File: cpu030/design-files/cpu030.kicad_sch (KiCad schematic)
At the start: 67 parts, among them J101 Reset, J102 SYSCTL JTAG, J103 NMI, SW101 Reset, SW102 NMI, U101 MC68030RC, U102 ATF1508AS, U103 74ACT05, U104 DS1813, U105 SST39SF040 (E), U106 SST39SF040 (O), U107 MC68882, U108 GAL22V10, U109 74ACT05, U110 DS1813, Y101 50MHz

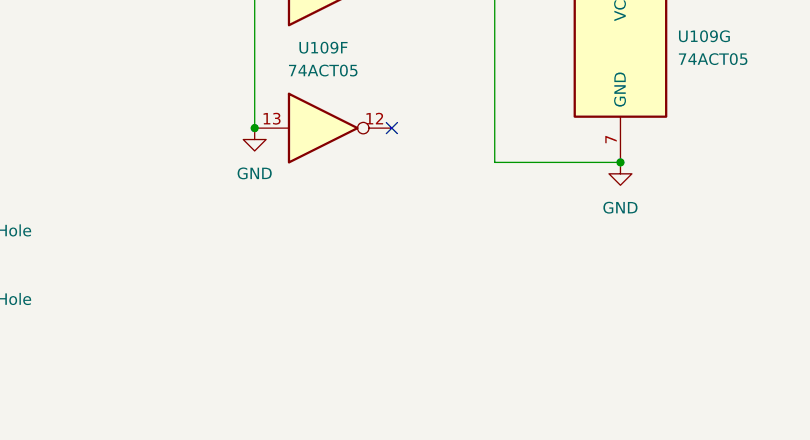
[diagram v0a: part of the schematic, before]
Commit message: Pullups on the INTx inputs.
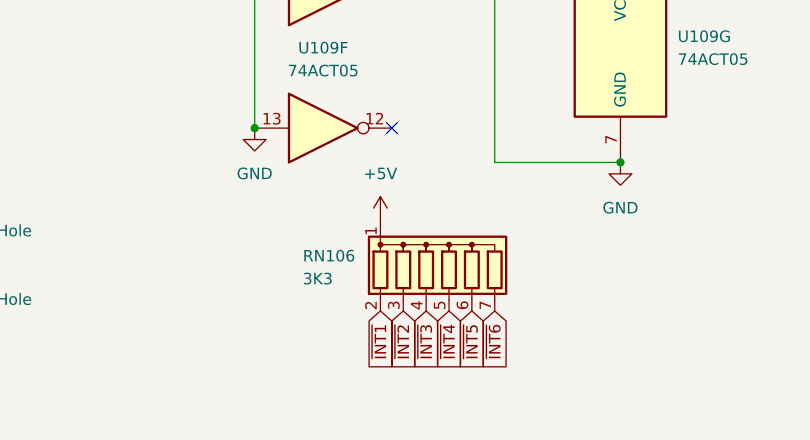
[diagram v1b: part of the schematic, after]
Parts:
- added RN106: 3K3, Resistor_THT:R_Array_SIP7, symbol Device:R_Network06
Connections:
- net +5V: now also RN106.1 (common)
- net ~{INT1}: now also RN106.2 (R1)
- net ~{INT2}: now also RN106.3 (R2)
- net ~{INT3}: now also RN106.4 (R3)
- net ~{INT4}: now also RN106.5 (R4)
- net ~{INT5}: now also RN106.6 (R5)
- net ~{INT6}: now also RN106.7 (R6)
